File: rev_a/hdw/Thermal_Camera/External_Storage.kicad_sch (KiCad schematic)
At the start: 38 parts

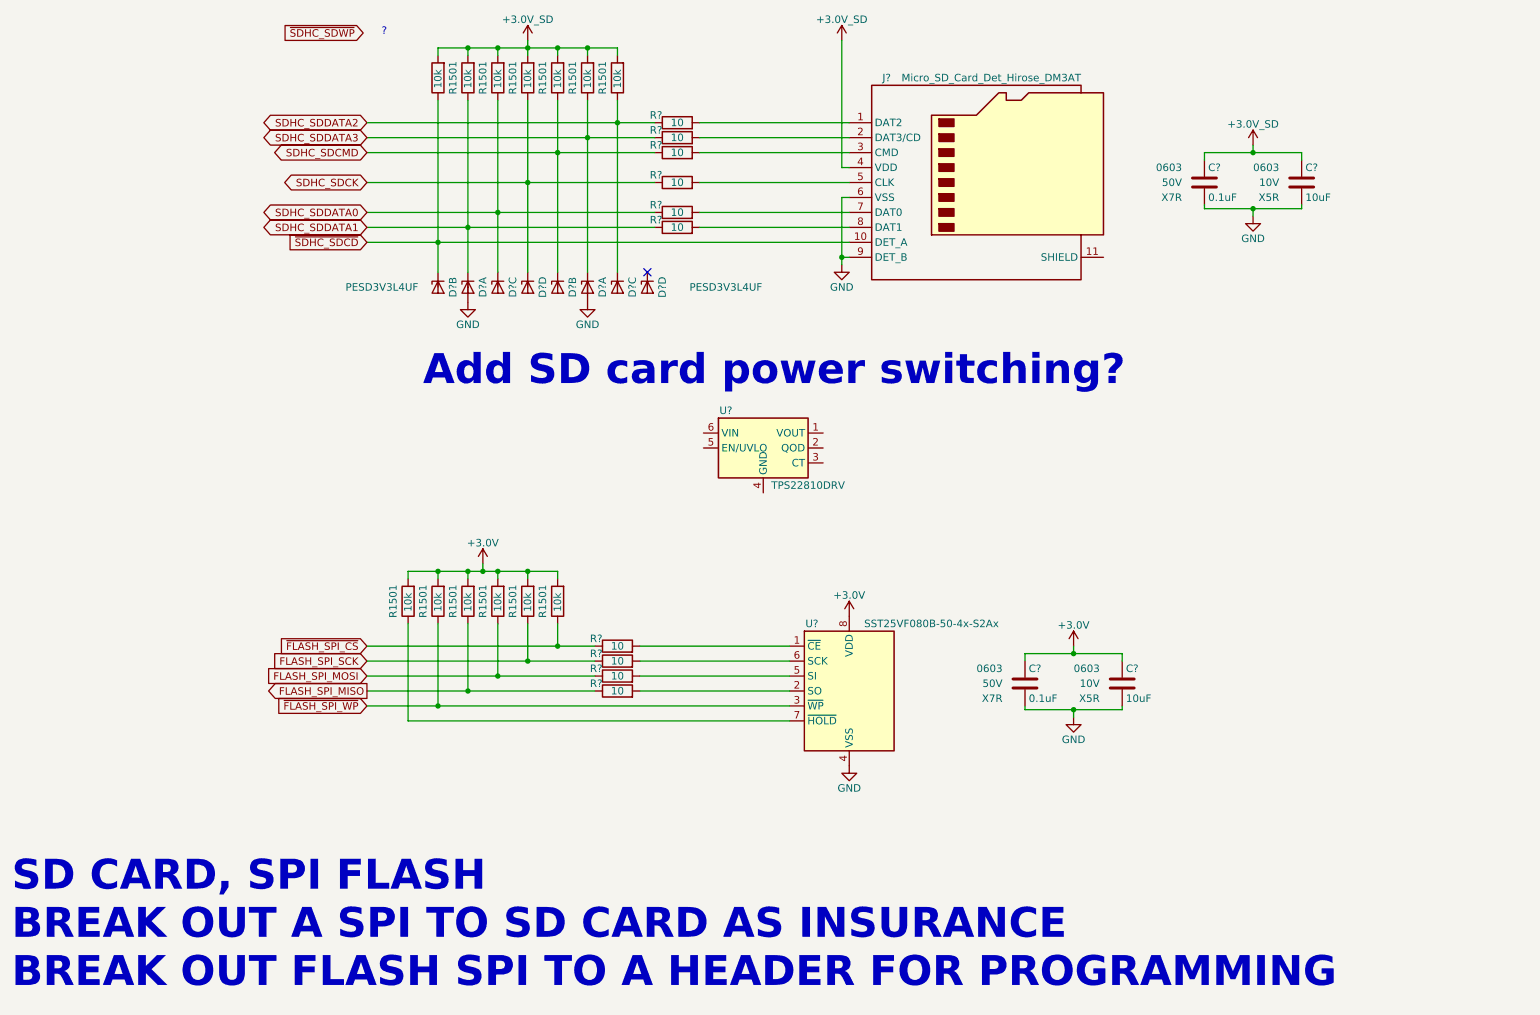
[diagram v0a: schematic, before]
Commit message: added PIC32 bypass, SD card load switch, other random junk
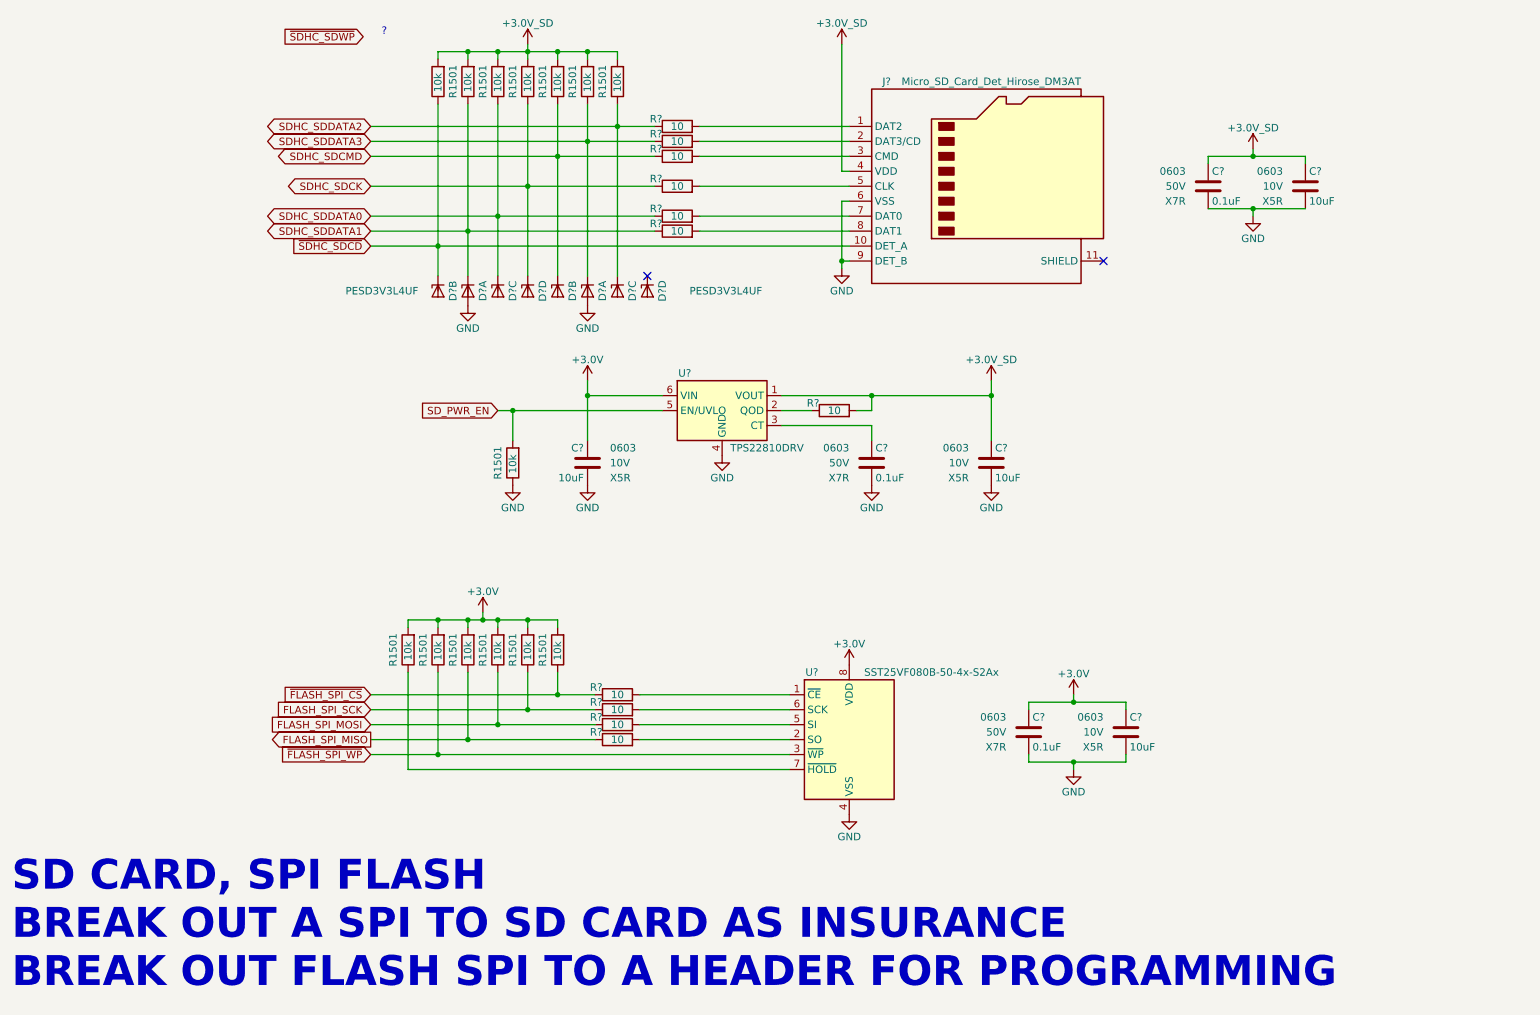
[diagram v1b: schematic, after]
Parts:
- added C?: 0.1uF, Capacitors_SMD:C_0603, symbol Custom_Library:C_Custom
- added C? (x2): 10uF, Capacitors_SMD:C_0603, symbol Custom_Library:C_Custom
- added R1501: 10k, Resistors_SMD:R_0603, symbol Custom_Library:R_Custom
- added R?: 10, Resistors_SMD:R_0603, symbol Custom_Library:R_Custom
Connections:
- net +3.0V: now also U?.6 (VIN), C?.1
- net +3.0V_SD: now also U?.1 (VOUT), C?.1, R?.1
- net GND: now also U?.4 (GND), U?.7 (GND), C?.2, C?.2, C?.2, R1501.2
- net at U?.2 (QOD): now also R?.2
- net at U?.3 (CT): now also C?.1
- net SD_PWR_EN: now reaches U?.5 (EN/UVLO)
- net SD_PWR_EN: now also R1501.1
- no-connect marks 1 -> 2
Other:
- note removed: "Add SD card power switching?"
- moved on the sheet: C?, D?A, D?B, D?C, D?D, J?, R1501, R?, U?
